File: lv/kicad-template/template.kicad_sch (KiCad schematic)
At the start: 1 part, among them U1 LM741

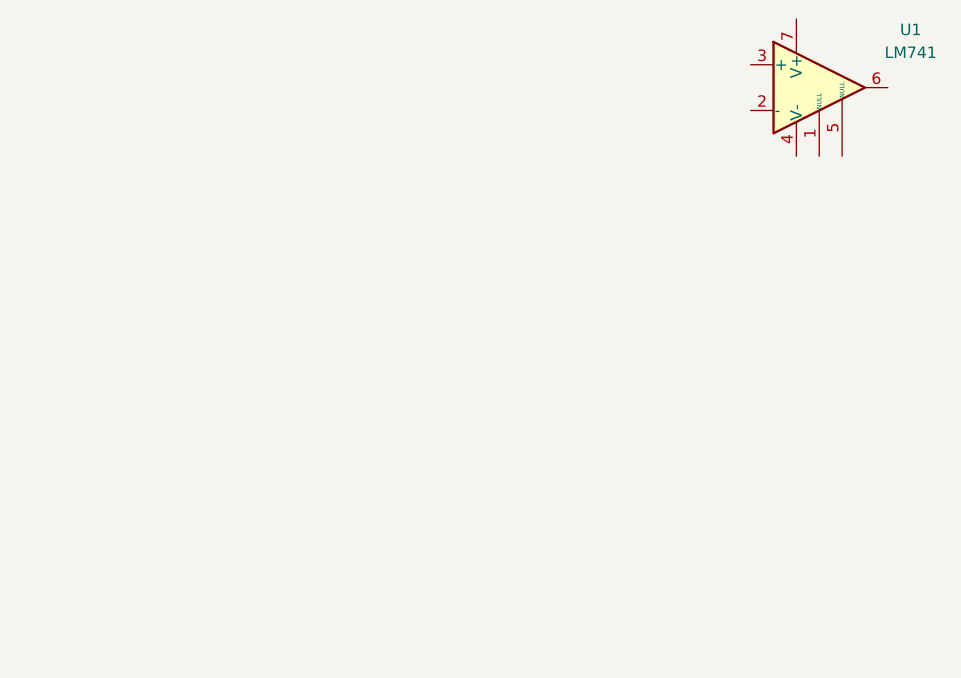
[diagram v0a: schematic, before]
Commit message: op amp succesful
Wasted a few hours making some goofy ah op amp that apperently wasn't an op amp, So I made a new one, its way more generic, hopefully its correct, was just making one before i started the bspd circuitboard, I ran an ac and dc test on its, seemed all good and what not.
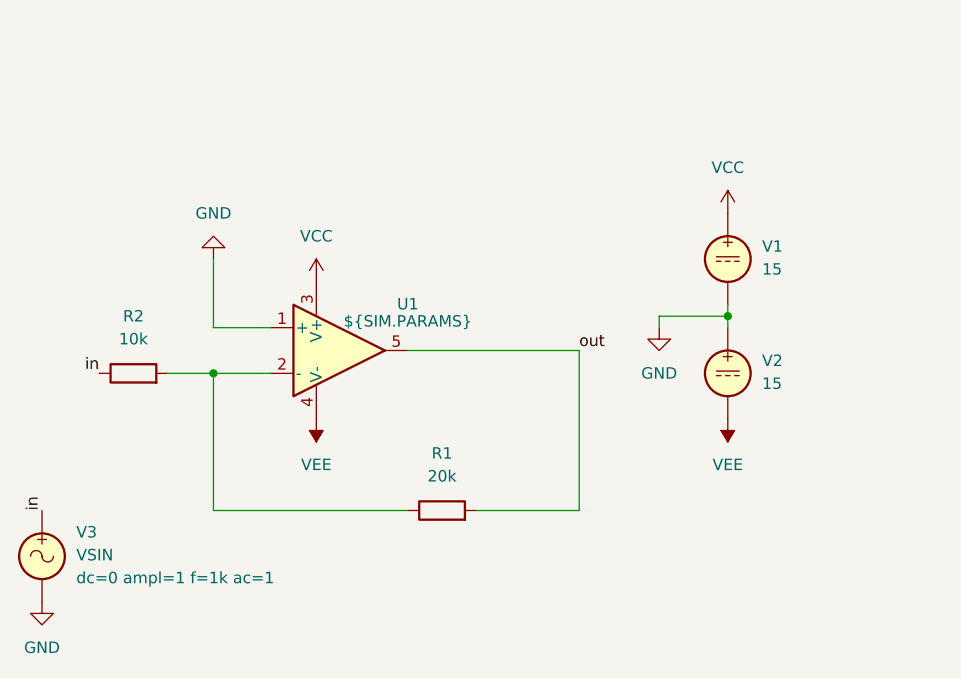
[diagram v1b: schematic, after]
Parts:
- removed U1: LM741, symbol Amplifier_Operational:LM741
- added R1: 20k, symbol Device:R
- added R2: 10k, symbol Device:R
- added U1: ${SIM.PARAMS}, symbol Simulation_SPICE:OPAMP
- added V1, V2: 15, symbol Simulation_SPICE:VDC
- added V3: VSIN, symbol Simulation_SPICE:VSIN
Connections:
- new net: R1.1, R2.2, U1.2 (-)
- new net GND: U1.1 (+), V1.2, V2.1, V3.2
- new net VCC: U1.3 (V+), V1.1
- new net VEE: U1.4 (V-), V2.2
- new net in: R2.1, V3.1
- new net out: R1.2, U1.5
